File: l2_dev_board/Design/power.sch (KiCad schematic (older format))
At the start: 50 parts, among them U1001 LT3480, U1002 NCP1529, U1003 NCP1529, U1004 NCP1529, U1005 APX803, U1006 NCP1529, U1007 NCP1529, U1008 APX803

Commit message: Started adding tracks
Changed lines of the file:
@@
-EESchema Schematic File Version 2  date 22/07/2011 14:08:59
+EESchema Schematic File Version 2  date 25/07/2011 13:55:09
 LIBS:power
 LIBS:device
@@
 LIBS:contrib
 LIBS:valves
-LIBS:LT3480
-LIBS:ncp1529
-LIBS:ncp303
-LIBS:nc7wz17
 LIBS:apx803
 LIBS:ase_20mhz
+LIBS:brooktre
+LIBS:cmos_ieee
 LIBS:Dmitri_Belimovl
 LIBS:EECV
+LIBS:elec-unifil
 LIBS:ft232r
+LIBS:gennum
+LIBS:graphic
+LIBS:LT3480
+LIBS:microchip1
+LIBS:nc7wz17
+LIBS:ncp303
+LIBS:ncp1529
+LIBS:pspice
 LIBS:SymbolsSimilarEN60617+oldDIN617
+LIBS:transf
+LIBS:ttl_ieee
+LIBS:video
 LIBS:xmos_capacitors
 LIBS:xmos_resistors
@@
 LIBS:xs1
 LIBS:XS1_L2_V2
-LIBS:L2DevBoard-cache
 EELAYER 25  0
 EELAYER END
@@
 Sheet 10 10
 Title ""
-Date "22 jul 2011"
+Date "25 jul 2011"
 Rev ""
 Comp ""
@@
 $EndDescr
 $Comp
-L +12V #PWR?
+L +12V #PWR038
 U 1 1 4E29763C
 P 650 650
-F 0 "#PWR?" H 650 600 20  0001 C CNN
+F 0 "#PWR038" H 650 600 20  0001 C CNN
 F 1 "+12V" H 650 750 30  0000 C CNN
 	1    650  650
@@
 $EndComp
 Wire Wire Line
-	1750 700  1200 700
-Wire Wire Line
-	1200 700  650  700
+	1750 700  650  700
 Wire Wire Line
 	650  700  650  650
@@
 Connection ~ 3850 5950
 Wire Wire Line
-	4050 5950 3850 5950
-Wire Wire Line
-	3850 5950 3550 5950
-Wire Wire Line
-	3550 5950 3300 5950
+	4050 5950 3300 5950
 Wire Wire Line
 	3300 5950 3300 6000
 Wire Wire Line
-	1200 5950 1050 5950
-Wire Wire Line
-	1050 5950 900  5950
+	1200 5950 900  5950
 Connection ~ 1050 5950
 Wire Wire Line
-	3550 6550 3300 6550
-Wire Wire Line
-	3300 6550 2700 6550
+	3550 6550 2700 6550
 Connection ~ 3300 6550
 Wire Wire Line
@@
 	3100 1400 2700 1400
 Wire Wire Line
-	2700 1400 2700 1600
-Wire Wire Line
-	2700 1600 2700 1750
+	2700 1400 2700 1750
 Wire Wire Line
 	1250 1550 800  1550
@@
 	800  1550 800  1600
 Wire Wire Line
-	650  2500 800  2500
-Wire Wire Line
-	800  2500 1100 2500
-Wire Wire Line
-	1100 2500 1950 2500
-Wire Wire Line
-	1950 2500 2800 2500
-Wire Wire Line
-	2800 2500 3400 2500
+	650  2500 3400 2500
 Connection ~ 2800 2000
 Wire Wire Line
-	2900 2000 2800 2000
-Wire Wire Line
-	2800 2000 2700 2000
+	2900 2000 2700 2000
 Wire Wire Line
 	7550 4950 7550 5050
 Connection ~ 7850 4450
 Wire Wire Line
-	8000 4450 7850 4450
-Wire Wire Line
-	7850 4450 7550 4450
-Wire Wire Line
-	7550 4450 7300 4450
+	8000 4450 7300 4450
 Wire Wire Line
 	7300 4450 7300 4500
@@
 	5200 5050 5050 5050
 Wire Wire Line
-	4900 4450 5050 4450
-Wire Wire Line
-	5050 4450 5200 4450
+	4900 4450 5200 4450
 Connection ~ 5050 4450
 Wire Wire Line
-	7550 5050 7300 5050
-Wire Wire Line
-	7300 5050 6700 5050
+	7550 5050 6700 5050
 Connection ~ 7300 5050
 Wire Wire Line
@@
 Connection ~ 7300 3550
 Wire Wire Line
-	6700 3550 7300 3550
-Wire Wire Line
-	7300 3550 7550 3550
+	6700 3550 7550 3550
 Connection ~ 5050 2950
 Wire Wire Line
-	4900 2950 5050 2950
-Wire Wire Line
-	5050 2950 5200 2950
+	4900 2950 5200 2950
 Wire Wire Line
 	5200 3550 5050 3550
@@
 	7300 3000 7300 2950
 Wire Wire Line
-	7300 2950 7550 2950
-Wire Wire Line
-	7550 2950 7850 2950
-Wire Wire Line
-	7850 2950 7950 2950
+	7300 2950 7950 2950
 Connection ~ 7850 2950
 Wire Wire Line
@@
 Connection ~ 3850 4450
 Wire Wire Line
-	4000 4450 3850 4450
-Wire Wire Line
-	3850 4450 3550 4450
-Wire Wire Line
-	3550 4450 3300 4450
+	4000 4450 3300 4450
 Wire Wire Line
 	3300 4450 3300 4500
@@
 	1200 5050 1100 5050
 Wire Wire Line
-	900  4450 1050 4450
-Wire Wire Line
-	1050 4450 1200 4450
+	900  4450 1200 4450
 Connection ~ 1050 4450
 Wire Wire Line
-	3550 5050 3300 5050
-Wire Wire Line
-	3300 5050 2700 5050
+	3550 5050 2700 5050
 Connection ~ 3300 5050
 Wire Wire Line
@@
 Connection ~ 3300 3550
 Wire Wire Line
-	2700 3550 3300 3550
-Wire Wire Line
-	3300 3550 3550 3550
+	2700 3550 3550 3550
 Connection ~ 1050 2950
 Wire Wire Line
-	3400 2000 3400 1600
-Wire Wire Line
-	3400 1600 3400 700
+	3400 2000 3400 700
 Connection ~ 2700 1600
 Connection ~ 1200 700
@@
 Connection ~ 3400 700
 Wire Wire Line
-	3450 700  3400 700
-Wire Wire Line
-	3400 700  2200 700
-Wire Wire Line
-	900  2950 1050 2950
-Wire Wire Line
-	1050 2950 1200 2950
+	3450 700  2200 700
+Wire Wire Line
+	900  2950 1200 2950
 Wire Wire Line
 	1200 3550 1100 3550
@@
 	3300 3000 3300 2950
 Wire Wire Line
-	3300 2950 3550 2950
-Wire Wire Line
-	3550 2950 3850 2950
-Wire Wire Line
-	3850 2950 4000 2950
+	3300 2950 4000 2950
 Connection ~ 3850 2950
 Wire Wire Line

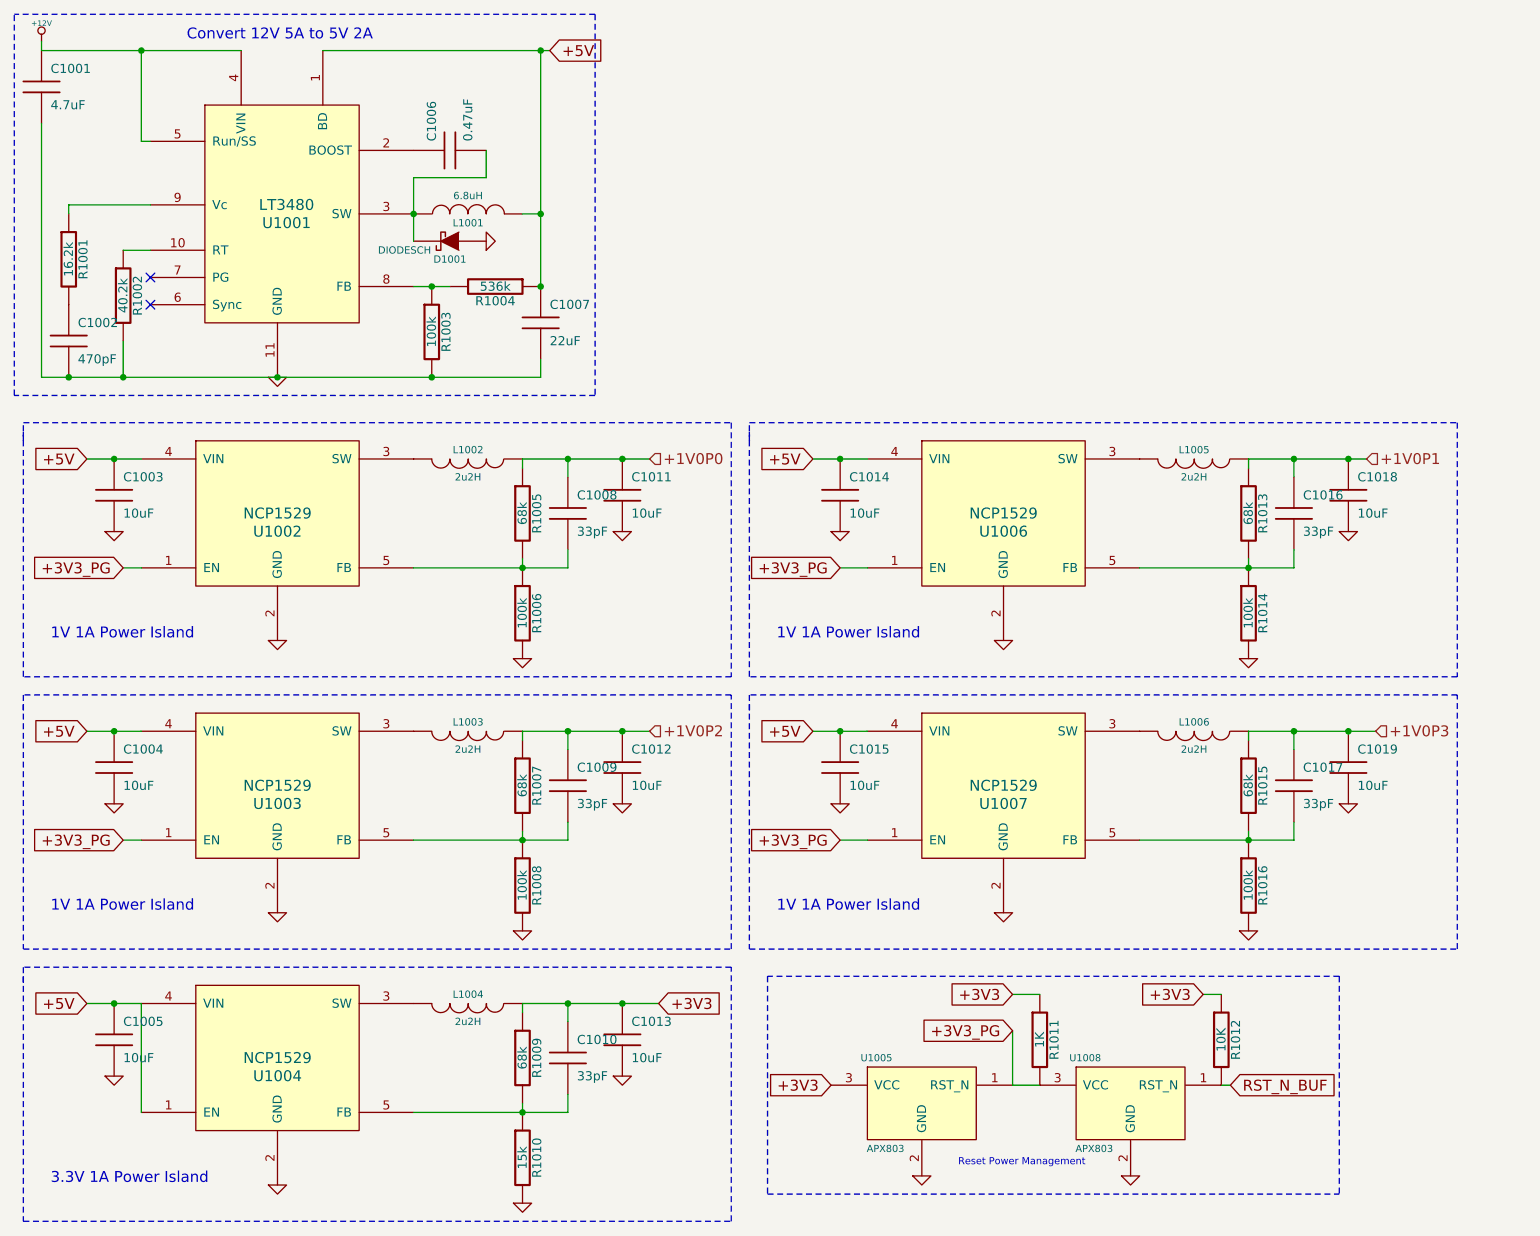
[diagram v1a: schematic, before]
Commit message: Added appropriate sepearte power modules. Moved buffering to hiearchial sheet Buffering per 2 L2s due to harsh pull down on pads moved pins from global labels to heirachial
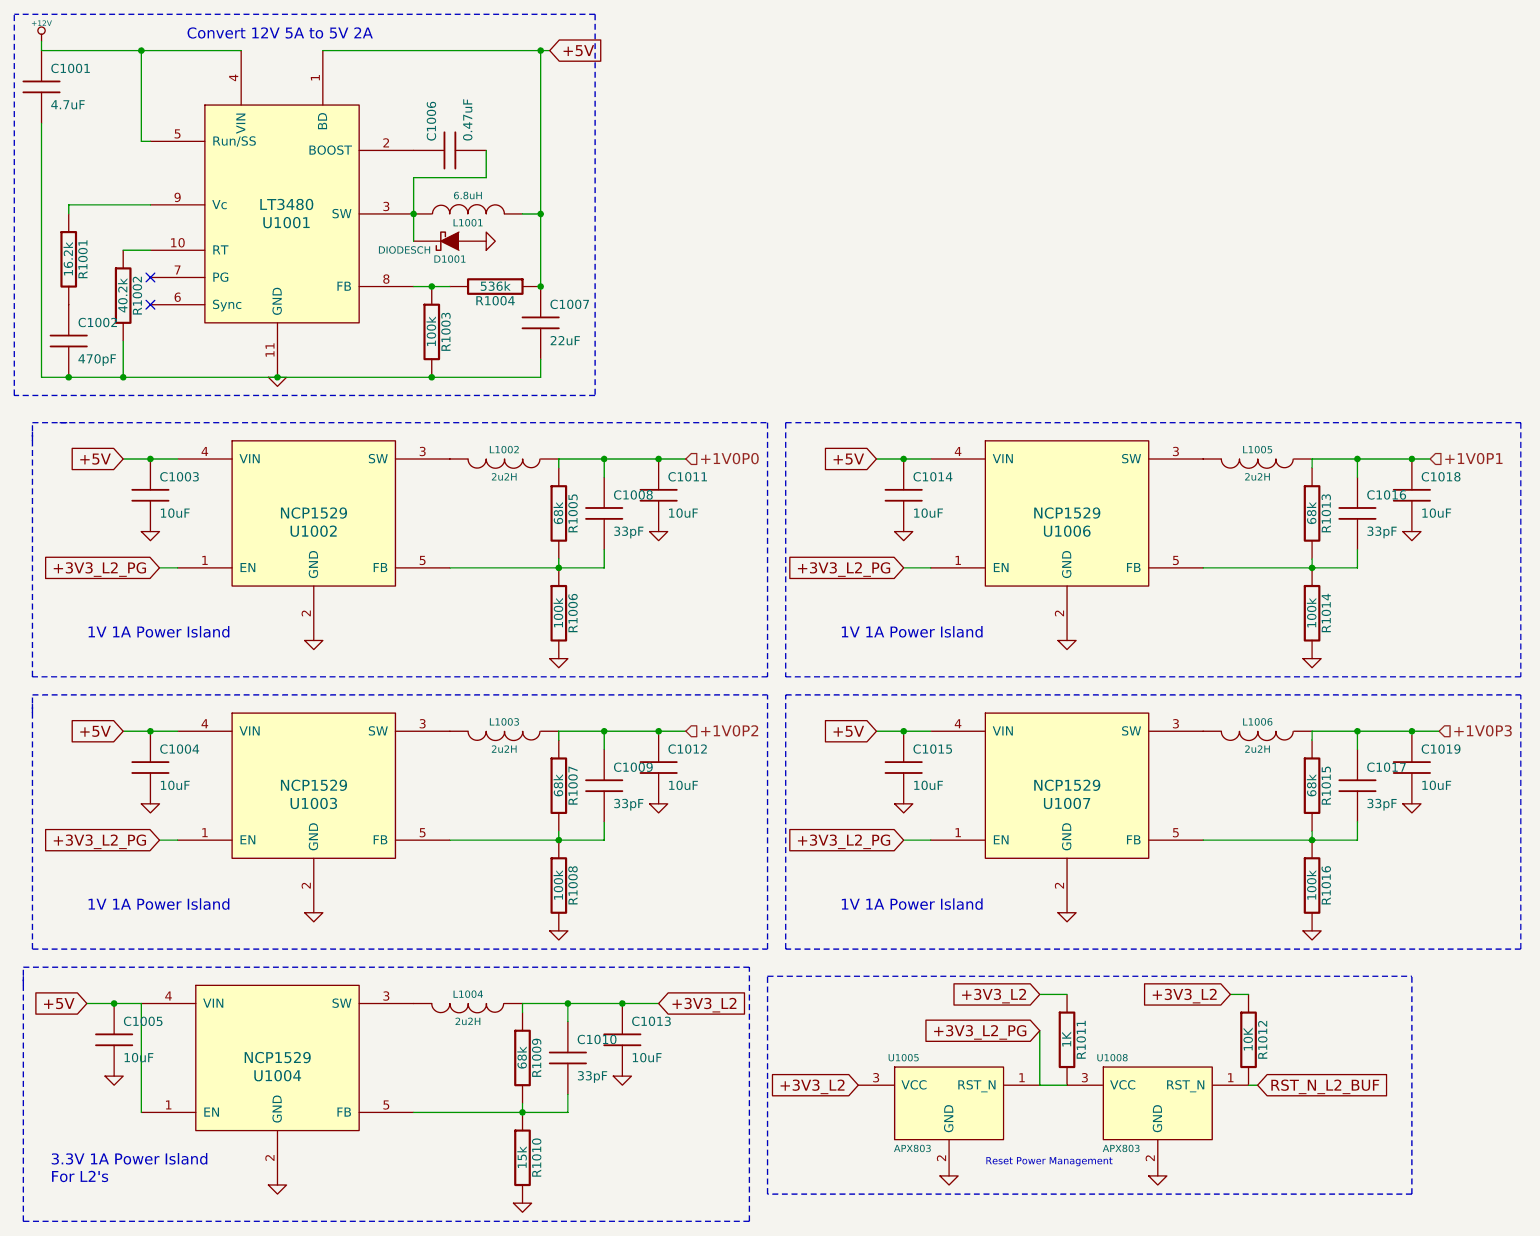
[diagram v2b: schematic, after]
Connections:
- net +3V3 renamed +3V3_L2
- net +3V3_PG renamed +3V3_L2_PG
- net RST_N_BUF renamed RST_N_L2_BUF
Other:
- note added: "3.3V 1A Power Island\nFor L2's"
- note removed: "3.3V 1A Power Island"
- moved on the sheet: C1003, C1004, C1008, C1009, C1011, C1012, C1014, C1015, C1016, C1017, C1018, C1019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
